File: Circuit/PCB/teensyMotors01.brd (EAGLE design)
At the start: 76.3 x 157.6 mm, 66 parts, among them SW1 219-10, U1 MUX-74HC4067

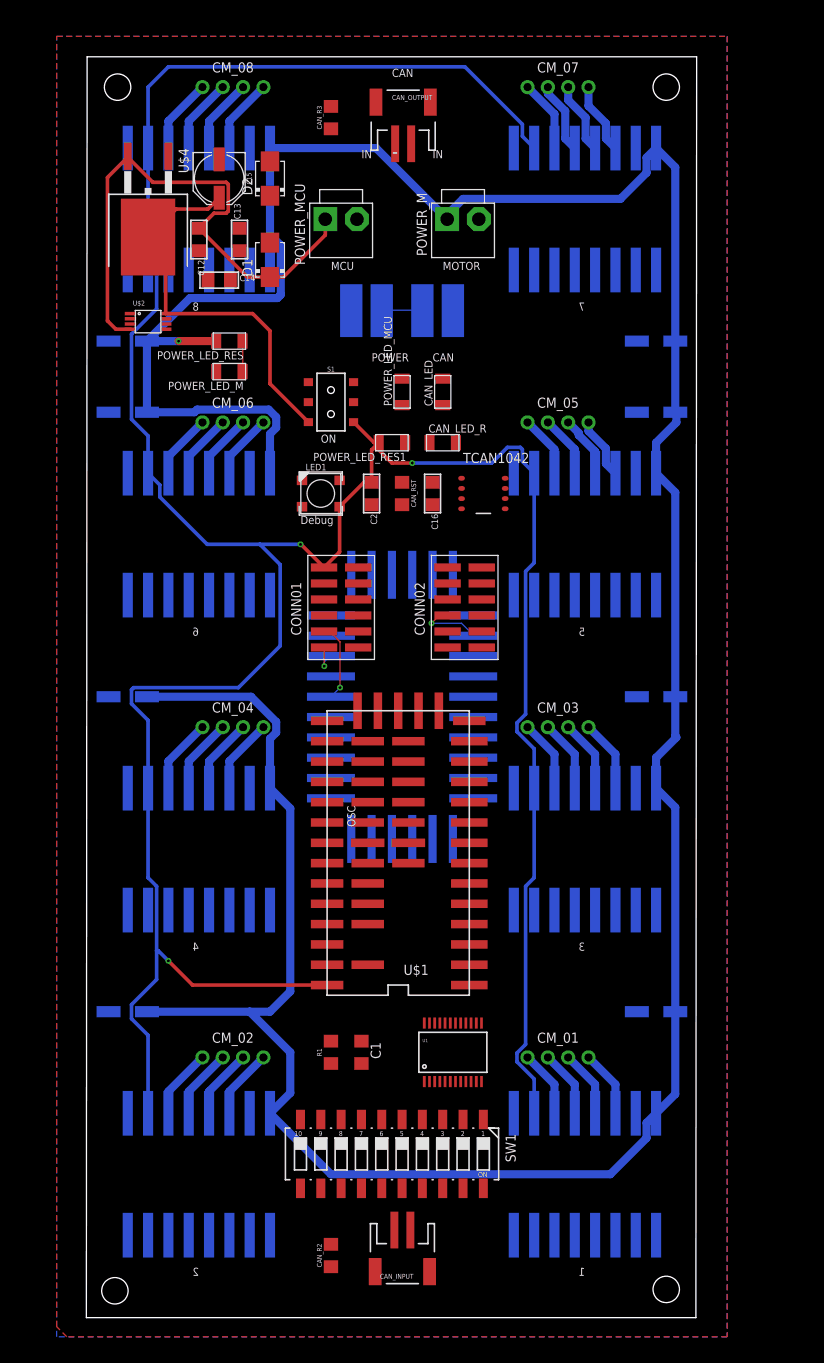
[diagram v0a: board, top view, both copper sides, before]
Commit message: updated main board
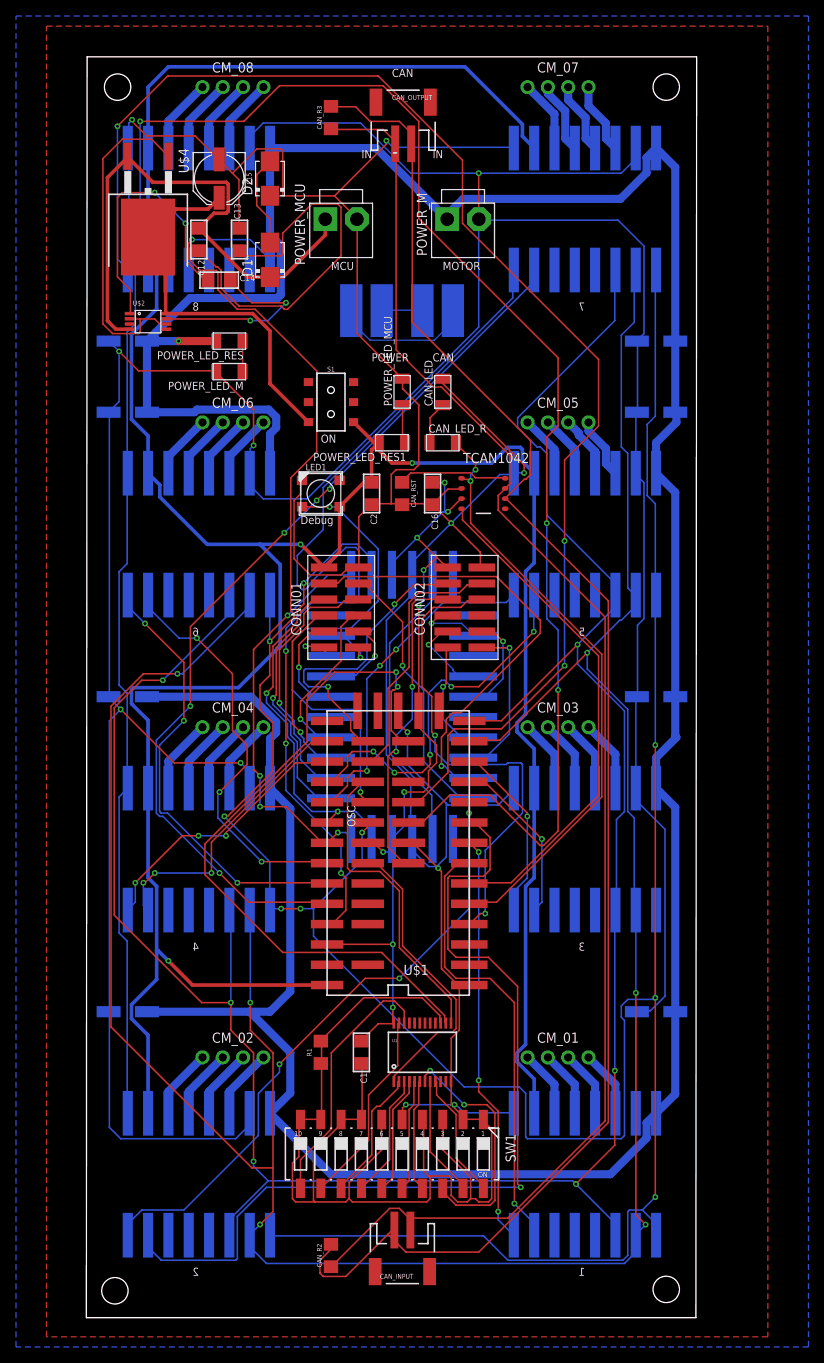
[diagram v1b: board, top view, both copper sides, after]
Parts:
- C1: value 0.1uF -> (none); device adafruit:C1206 -> microbuilder:1206
- moved U1 3.81 mm to (43.2, 34.3)
- moved R1 1.27 mm to (30.5, 34.3)
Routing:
- net GND_MCU: track 0.00 -> 599.1 mm, vias 0 -> 8
- net GND_M: track 0.00 -> 420.2 mm, vias 0 -> 5
- net MENABLE: track 0.00 -> 404.0 mm, vias 0 -> 9
- net MMS1: track 0.00 -> 335.7 mm, vias 0 -> 6
- net MMS2: track 0.00 -> 307.5 mm, vias 0 -> 6
- net CAN_L: track 0.00 -> 199.4 mm
- net CAN_H: track 0.00 -> 190.0 mm
- net MSTEP_08: track 0.00 -> 178.1 mm, vias 0 -> 3
- net MDIR_08: track 0.00 -> 169.9 mm, vias 0 -> 3
- net MDIR_07: track 0.00 -> 119.1 mm, vias 0 -> 3
- net MSTEP_07: track 0.00 -> 113.7 mm, vias 0 -> 5
- net MSTEP_02: track 0.00 -> 113.5 mm, vias 0 -> 1
- net 3.3V: track 0.00 -> 106.5 mm, vias 0 -> 9
- net MUX_S2: track 0.00 -> 88.5 mm, vias 0 -> 2
- net MDIR_02: track 0.00 -> 77.4 mm, vias 0 -> 3
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- added copper zone on layer 16, net GND_MCU
- removed copper zone on layer 16, net GND_M
